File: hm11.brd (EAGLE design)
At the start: 17.2 x 18 mm, 3 parts

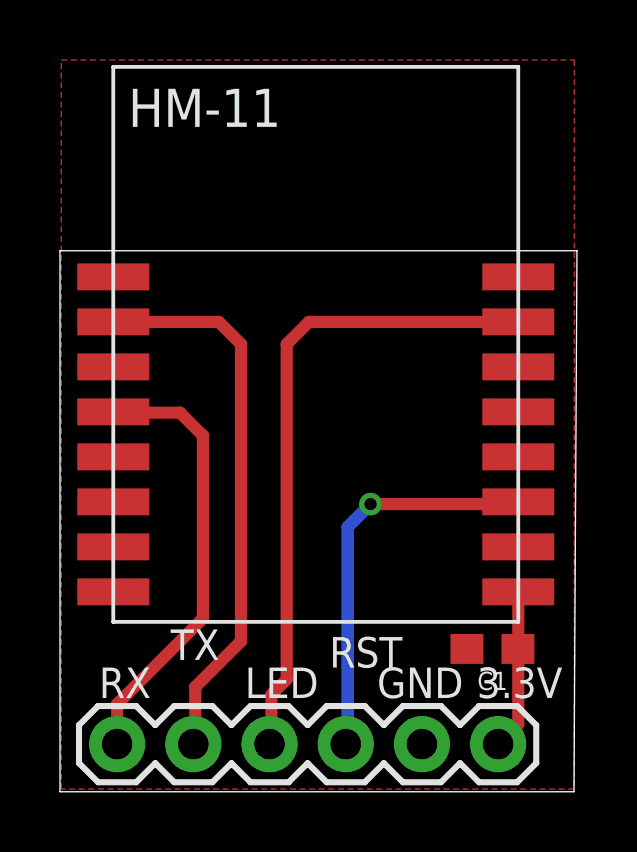
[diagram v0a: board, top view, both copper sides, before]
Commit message: update traces
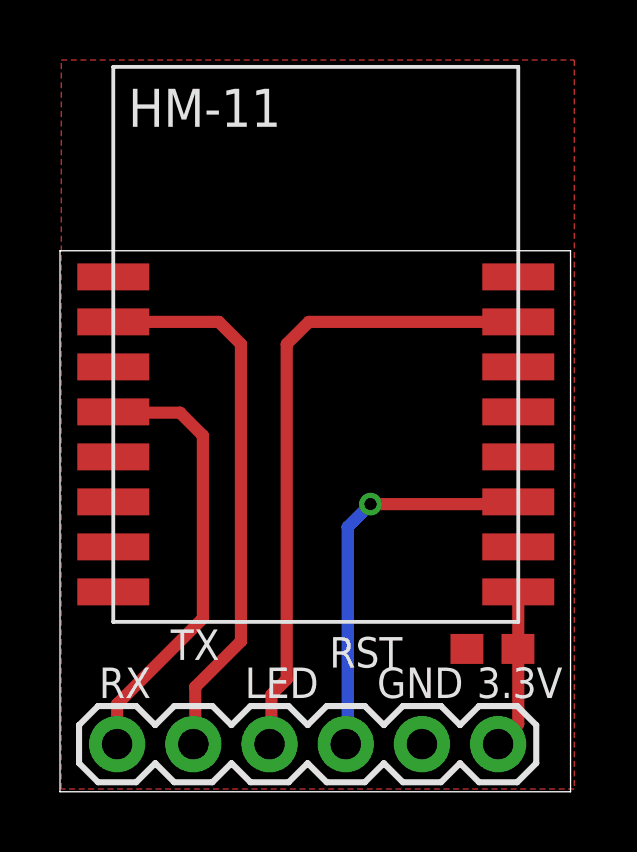
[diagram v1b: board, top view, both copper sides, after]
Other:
- board size 17.2 x 18 mm -> 17 x 18 mm
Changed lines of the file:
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@@
 <layer number="23" name="tOrigins" color="15" fill="1" visible="yes" active="yes"/>
 <layer number="24" name="bOrigins" color="15" fill="1" visible="yes" active="yes"/>
-<layer number="25" name="tNames" color="7" fill="1" visible="no" active="yes"/>
-<layer number="26" name="bNames" color="7" fill="1" visible="no" active="yes"/>
-<layer number="27" name="tValues" color="7" fill="1" visible="no" active="yes"/>
-<layer number="28" name="bValues" color="7" fill="1" visible="no" active="yes"/>
-<layer number="29" name="tStop" color="7" fill="3" visible="yes" active="yes"/>
-<layer number="30" name="bStop" color="7" fill="6" visible="yes" active="yes"/>
+<layer number="25" name="tNames" color="7" fill="1" visible="yes" active="yes"/>
+<layer number="26" name="bNames" color="7" fill="1" visible="yes" active="yes"/>
+<layer number="27" name="tValues" color="7" fill="1" visible="yes" active="yes"/>
+<layer number="28" name="bValues" color="7" fill="1" visible="yes" active="yes"/>
+<layer number="29" name="tStop" color="7" fill="3" visible="no" active="yes"/>
+<layer number="30" name="bStop" color="7" fill="6" visible="no" active="yes"/>
 <layer number="31" name="tCream" color="7" fill="4" visible="no" active="yes"/>
 <layer number="32" name="bCream" color="7" fill="5" visible="no" active="yes"/>
@@
 <board>
 <plain>
-<wire x1="28.2575" y1="21.9075" x2="45.39" y2="21.9075" width="0" layer="20"/>
-<wire x1="45.39" y1="21.9075" x2="45.49" y2="39.9415" width="0" layer="20"/>
-<wire x1="45.49" y1="39.9415" x2="28.2575" y2="39.9415" width="0" layer="20"/>
+<wire x1="28.2575" y1="21.9075" x2="45.2755" y2="21.9075" width="0" layer="20"/>
+<wire x1="45.2755" y1="21.9075" x2="45.2755" y2="39.9415" width="0" layer="20"/>
+<wire x1="45.2755" y1="39.9415" x2="28.2575" y2="39.9415" width="0" layer="20"/>
 <wire x1="28.2575" y1="39.9415" x2="28.2575" y2="21.9075" width="0" layer="20"/>
 <text x="31.288" y="26.048" size="1.016" layer="21" font="vector" ratio="15" rot="R180">RX</text>
@@
 <attribute name="VALUE" x="44.1325" y="26.67" size="1.27" layer="27" rot="R180"/>
 </element>
-<element name="C1" library="SparkFun-Capacitors" package="0603" value="1.0uF" x="42.672" y="26.67" rot="R180">
+<element name="C1" library="SparkFun-Capacitors" package="0603" value="1.0uF" x="42.672" y="26.67" smashed="yes" rot="R180">
 <attribute name="PROD_ID" value="CAP-00868" x="42.672" y="26.67" size="1.778" layer="27" font="vector" ratio="15" rot="R180" display="off"/>
+<attribute name="VALUE" x="42.672" y="27.432" size="0.6096" layer="27" font="vector" ratio="20" rot="R180" align="top-center"/>
 </element>
 </elements>
